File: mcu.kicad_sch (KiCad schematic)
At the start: 14 parts

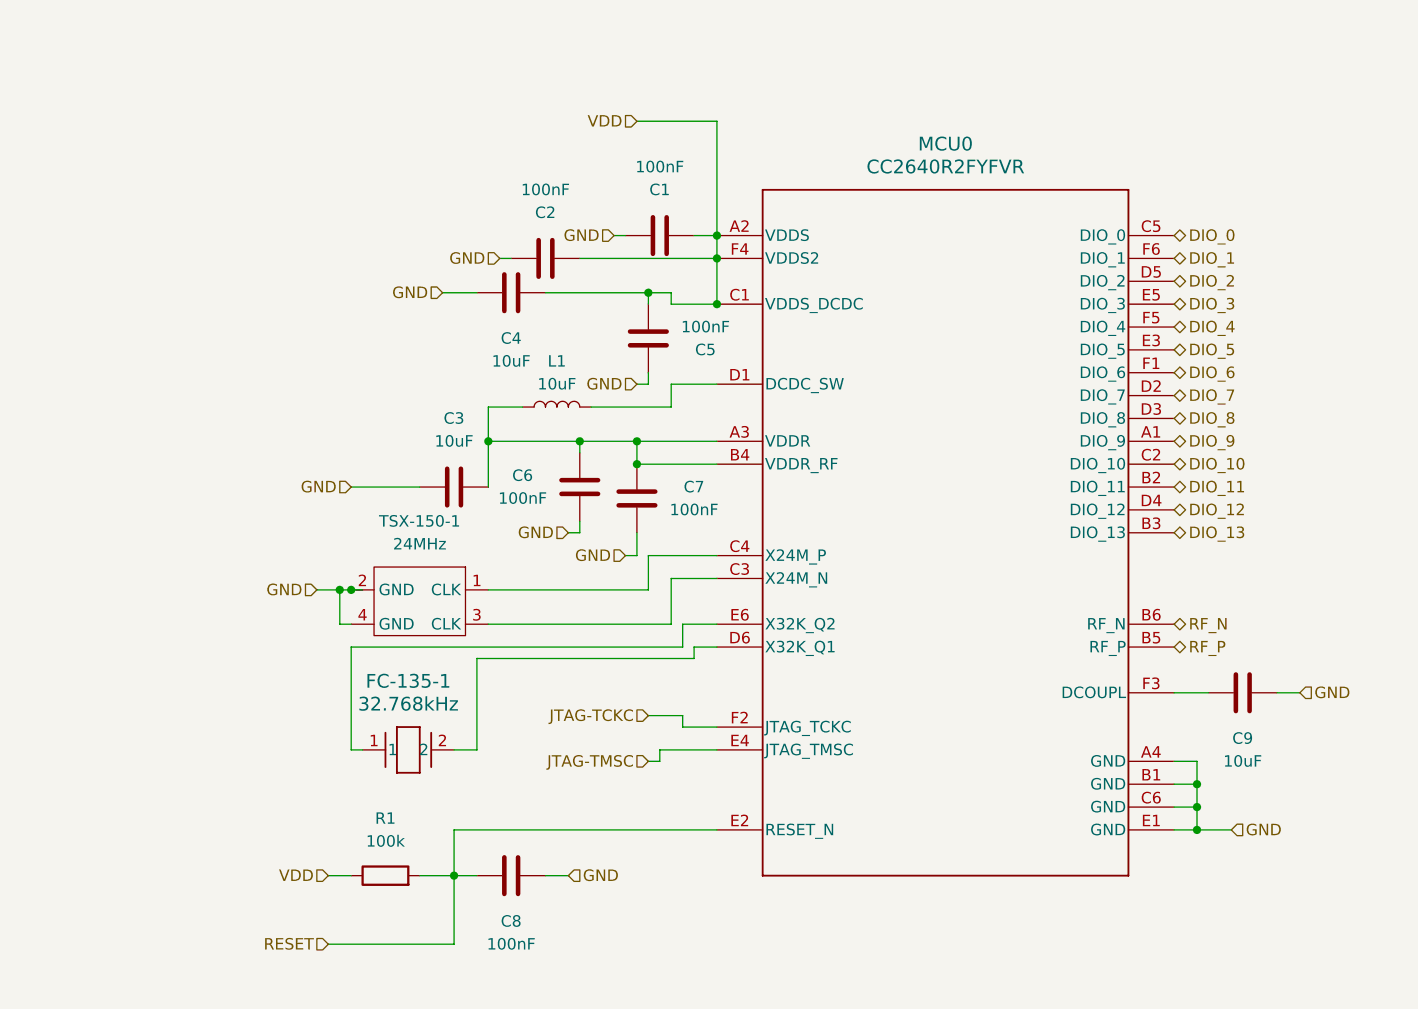
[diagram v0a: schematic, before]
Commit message: schematic 90%
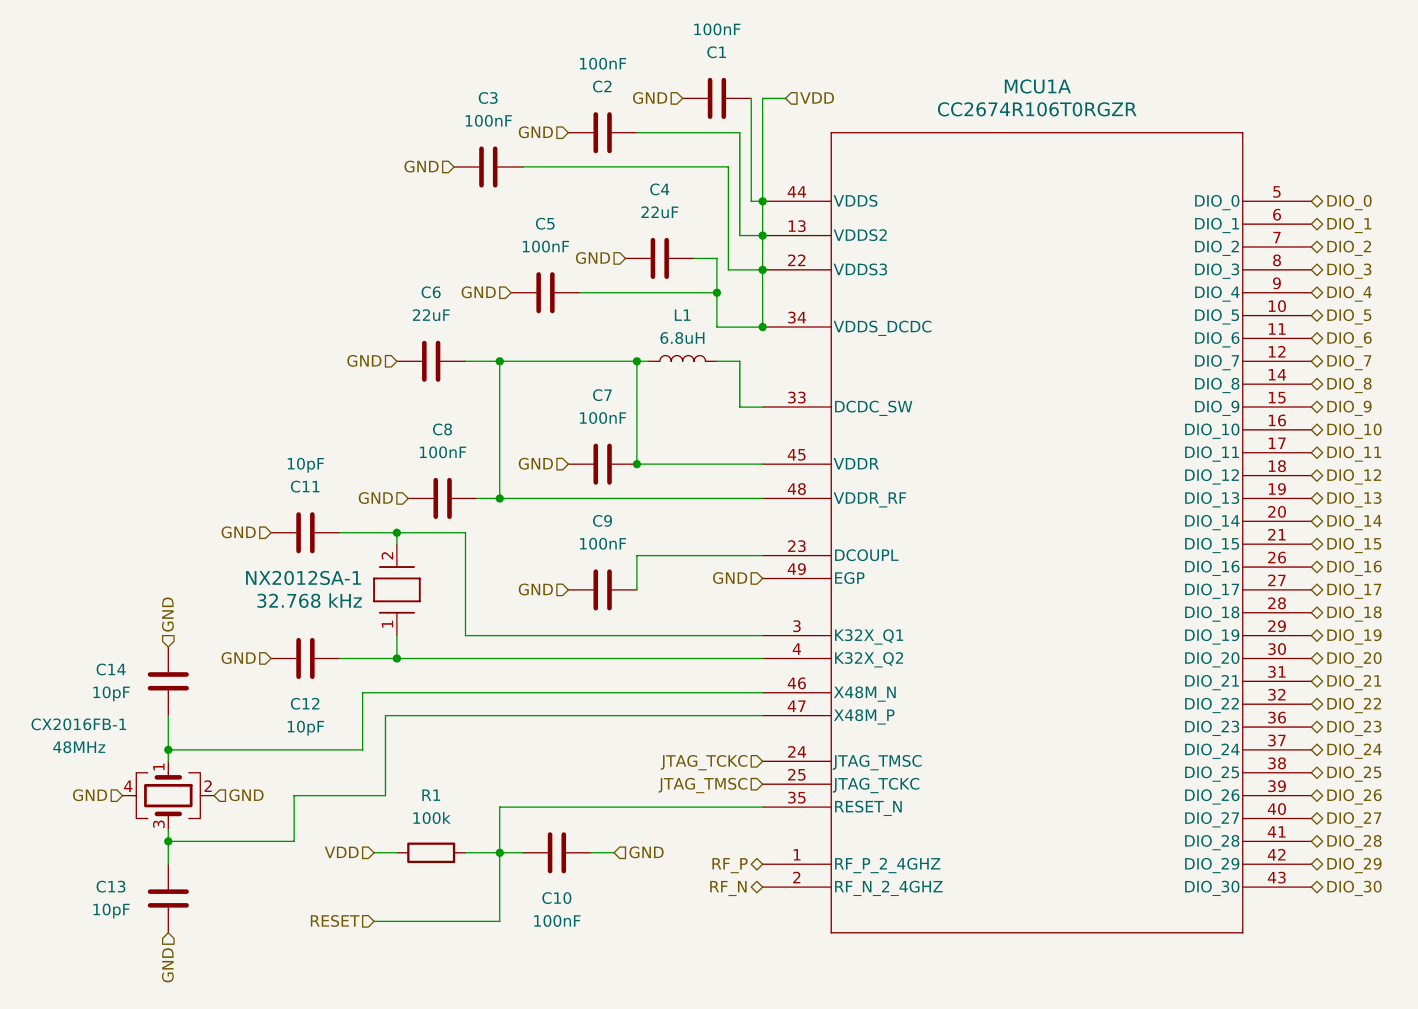
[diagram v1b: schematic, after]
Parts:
- removed C3: 10uF, Capacitor_SMD:C_0805_2012Metric, symbol Device:C
- removed FC-135-1: 32.768kHz, XTAL_FC-135_EPS, symbol ProjectSymbols:FC-135_32.7680KA-A5
- removed MCU0: CC2640R2FYFVR, YFV0034ALAL, symbol ProjectSymbols:CC2640R2FYFVR
- removed TSX-150-1: 24MHz, symbol ProjectSymbols:TSX-3225
- added C11, C12, C13, C14: 10pF, Capacitor_SMD:C_1206_3216Metric, symbol Device:C
- added C5: 100nF, Capacitor_SMD:C_1206_3216Metric, symbol Device:C
- added C6: 22uF, Capacitor_SMD:C_0805_2012Metric, symbol Device:C
- added CX2016FB-1: 48MHz, Crystal:Crystal_SMD_2016-4Pin_2.0x1.6mm, symbol Device:Crystal_GND24
- added MCU1: CC2674R106T0RGZR, VQFN48_RGZ_TEX, symbol ProjectSymbols:CC2674R106T0RGZR
- added NX2012SA-1: 32.768 kHz, Crystal:Crystal_SMD_2012-2Pin_2.0x1.2mm, symbol ProjectSymbols:FC-135_32.7680KA-A5
- C4: value 10uF -> 22uF
- C9: value 10uF -> 100nF; footprint Capacitor_SMD:C_0805_2012Metric -> Capacitor_SMD:C_1206_3216Metric
- L1: value 10uF -> 6.8uH
- renumbered C8 to C10, C5 to C3, C6 to C8
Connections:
- net DIO_0: now also MCU1.5 (DIO_0)
- net DIO_1: now also MCU1.6 (DIO_1)
- net DIO_10: now also MCU1.16 (DIO_10)
- net DIO_11: now also MCU1.17 (DIO_11)
- net DIO_12: now also MCU1.18 (DIO_12)
- net DIO_13: now also MCU1.19 (DIO_13)
- net DIO_2: now also MCU1.7 (DIO_2)
- net DIO_3: now also MCU1.8 (DIO_3)
- net DIO_4: now also MCU1.9 (DIO_4)
- net DIO_5: now also MCU1.10 (DIO_5)
- net DIO_6: now also MCU1.11 (DIO_6)
- net DIO_7: now also MCU1.12 (DIO_7)
- net DIO_8: now also MCU1.14 (DIO_8)
- net DIO_9: now also MCU1.15 (DIO_9)
- net GND: now also C3.2, C4.1, C7.2, C9.2, C11.2, C12.1, C13.2, C14.1, C5.2, C6.1, CX2016FB-1.2, CX2016FB-1.4, MCU1.49 (EGP); no longer C3.1, C4.2, C7.1, C9.1
- net RESET: now also MCU1.35 (RESET_N)
- net RF_N: now also MCU1.2 (RF_N_2_4GHZ)
- net RF_P: now also MCU1.1 (RF_P_2_4GHZ)
- net VDD: now also C3.1, C4.2, C5.1, MCU1.13 (VDDS2), MCU1.22 (VDDS3), MCU1.34 (VDDS_DCDC), MCU1.44 (VDDS); no longer C3.2, C4.1
- net at C8.1, L1.1: now also C7.1, C6.2, MCU1.45 (VDDR), MCU1.48 (VDDR_RF); no longer C7.2
- net at L1.2: now also MCU1.33 (DCDC_SW)
- new net: C14.2, CX2016FB-1.1, MCU1.46 (X48M_N)
- new net: C13.1, CX2016FB-1.3, MCU1.47 (X48M_P)
- new net: C12.2, MCU1.4 (K32X_Q2), NX2012SA-1.1
- new net: C9.1, MCU1.23 (DCOUPL)
- new net: C11.1, MCU1.3 (K32X_Q1), NX2012SA-1.2
- new net DIO_14: MCU1.20 (DIO_14)
- new net DIO_15: MCU1.21 (DIO_15)
- new net DIO_16: MCU1.26 (DIO_16)
- new net DIO_17: MCU1.27 (DIO_17)
- new net DIO_18: MCU1.28 (DIO_18)
- new net DIO_19: MCU1.29 (DIO_19)
- new net DIO_20: MCU1.30 (DIO_20)
- new net DIO_21: MCU1.31 (DIO_21)
- new net DIO_22: MCU1.32 (DIO_22)
- new net DIO_23: MCU1.36 (DIO_23)
- new net DIO_24: MCU1.37 (DIO_24)
- new net DIO_25: MCU1.38 (DIO_25)
- new net DIO_26: MCU1.39 (DIO_26)
- new net DIO_27: MCU1.40 (DIO_27)
- new net DIO_28: MCU1.41 (DIO_28)
- new net DIO_29: MCU1.42 (DIO_29)
- new net DIO_30: MCU1.43 (DIO_30)
- new net JTAG_TCKC: MCU1.24 (JTAG_TMSC)
- new net JTAG_TMSC: MCU1.25 (JTAG_TCKC)
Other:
- moved on the sheet: C1, C10, C2, C3, C4, C7, C8, L1, R1
